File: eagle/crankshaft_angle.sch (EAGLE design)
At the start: 2 parts, among them U1 ATTINY25V-10PU

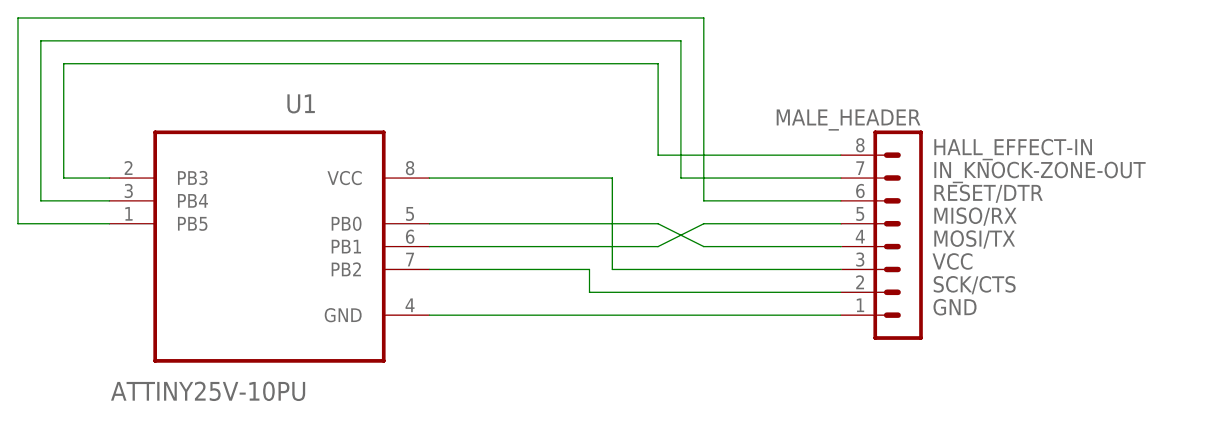
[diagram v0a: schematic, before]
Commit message: edit schematics
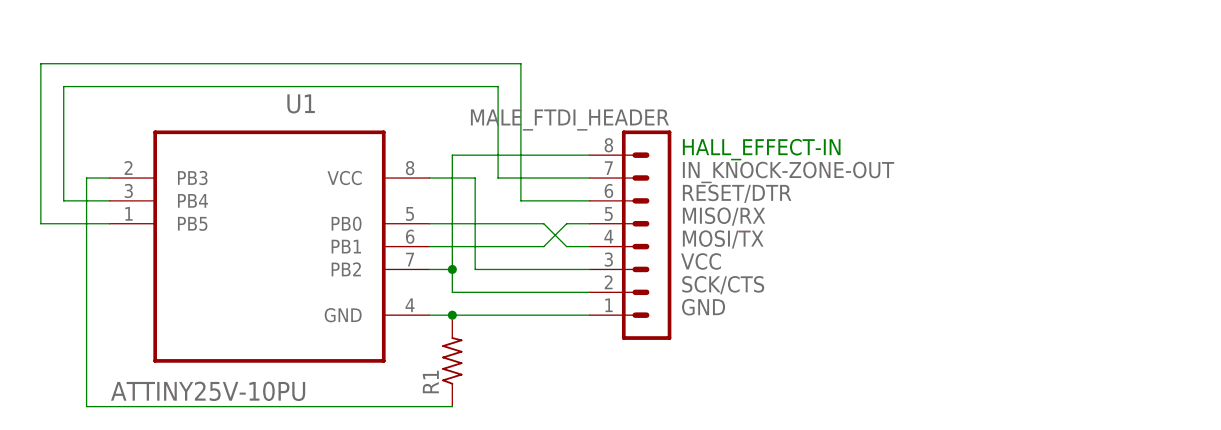
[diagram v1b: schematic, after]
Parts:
- removed MALE_HEADER: (no value), con-lstb:MA08-1
- added MALE_FTDI_HEADER: (no value), con-lstb:MA08-1
- added R1: (no value), rcl:R-US_0204/7
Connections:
- removed net HALL_EFFECT-IN: MALE_HEADER.8, U1.PB3
- new net N$1: R1.1, U1.PB3
- net GND: now also MALE_FTDI_HEADER.1, R1.2; no longer MALE_HEADER.1
- net IN_KNOCK-ZONE-OUT: now also MALE_FTDI_HEADER.7; no longer MALE_HEADER.7
- net MISO/RX: now also MALE_FTDI_HEADER.5; no longer MALE_HEADER.5
- net MOSI/TX: now also MALE_FTDI_HEADER.4; no longer MALE_HEADER.4
- net RESET/DTR: now also MALE_FTDI_HEADER.6; no longer MALE_HEADER.6
- net SCK/CTS: now also MALE_FTDI_HEADER.2, MALE_FTDI_HEADER.8; no longer MALE_HEADER.2
- net VCC: now also MALE_FTDI_HEADER.3; no longer MALE_HEADER.3
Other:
- note added: "HALL_EFFECT-IN"
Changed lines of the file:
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@@
 <part name="FRAME1" library="frames" deviceset="LETTER_L" device=""/>
 <part name="U1" library="Atmel_By_element14_Batch_1-00" deviceset="ATTINY25V-10PU" device=""/>
-<part name="MALE_HEADER" library="con-lstb" deviceset="MA08-1" device=""/>
+<part name="MALE_FTDI_HEADER" library="con-lstb" deviceset="MA08-1" device=""/>
+<part name="R1" library="rcl" deviceset="R-US_" device="0204/7"/>
 </parts>
 <sheets>
 <sheet>
 <plain>
+<text x="152.4" y="81.28" size="1.778" layer="91">HALL_EFFECT-IN</text>
 </plain>
 <instances>
@@
 <instance part="FRAME1" gate="G$2" x="139.7" y="-17.78"/>
 <instance part="U1" gate="A" x="106.68" y="73.66" rot="MR0"/>
-<instance part="MALE_HEADER" gate="1" x="177.8" y="71.12" rot="MR0"/>
+<instance part="MALE_FTDI_HEADER" gate="1" x="149.86" y="71.12" rot="MR0"/>
+<instance part="R1" gate="G$1" x="127" y="58.42" rot="R90"/>
 </instances>
 <busses>
@@
 <net name="SCK/CTS" class="0">
 <segment>
-<wire x1="170.18" y1="66.04" x2="142.24" y2="66.04" width="0.1524" layer="91"/>
-<wire x1="142.24" y1="66.04" x2="142.24" y2="68.58" width="0.1524" layer="91"/>
+<pinref part="MALE_FTDI_HEADER" gate="1" pin="8"/>
 <pinref part="U1" gate="A" pin="PB2"/>
-<wire x1="142.24" y1="68.58" x2="124.46" y2="68.58" width="0.1524" layer="91"/>
-<pinref part="MALE_HEADER" gate="1" pin="2"/>
-<label x="180.34" y="66.04" size="1.778" layer="95"/>
+<wire x1="127" y1="68.58" x2="124.46" y2="68.58" width="0.1524" layer="91"/>
+<wire x1="142.24" y1="81.28" x2="127" y2="81.28" width="0.1524" layer="91"/>
+<wire x1="127" y1="81.28" x2="127" y2="68.58" width="0.1524" layer="91"/>
+<wire x1="127" y1="68.58" x2="127" y2="66.04" width="0.1524" layer="91"/>
+<junction x="127" y="68.58"/>
+<pinref part="MALE_FTDI_HEADER" gate="1" pin="2"/>
+<wire x1="127" y1="66.04" x2="142.24" y2="66.04" width="0.1524" layer="91"/>
+<label x="152.4" y="66.04" size="1.778" layer="95"/>
 </segment>
 </net>
 <net name="RESET/DTR" class="0">
 <segment>
-<wire x1="154.94" y1="76.2" x2="154.94" y2="96.52" width="0.1524" layer="91"/>
-<wire x1="154.94" y1="96.52" x2="78.74" y2="96.52" width="0.1524" layer="91"/>
-<wire x1="78.74" y1="96.52" x2="78.74" y2="73.66" width="0.1524" layer="91"/>
+<wire x1="134.62" y1="76.2" x2="134.62" y2="91.44" width="0.1524" layer="91"/>
+<wire x1="134.62" y1="91.44" x2="81.28" y2="91.44" width="0.1524" layer="91"/>
+<wire x1="81.28" y1="91.44" x2="81.28" y2="73.66" width="0.1524" layer="91"/>
 <pinref part="U1" gate="A" pin="PB5"/>
-<wire x1="78.74" y1="73.66" x2="88.9" y2="73.66" width="0.1524" layer="91"/>
-<pinref part="MALE_HEADER" gate="1" pin="6"/>
-<wire x1="170.18" y1="76.2" x2="154.94" y2="76.2" width="0.1524" layer="91"/>
-<label x="180.34" y="76.2" size="1.778" layer="95"/>
+<wire x1="81.28" y1="73.66" x2="88.9" y2="73.66" width="0.1524" layer="91"/>
+<pinref part="MALE_FTDI_HEADER" gate="1" pin="6"/>
+<wire x1="142.24" y1="76.2" x2="134.62" y2="76.2" width="0.1524" layer="91"/>
+<label x="152.4" y="76.2" size="1.778" layer="95"/>
 </segment>
 </net>
@@
 <segment>
 <pinref part="U1" gate="A" pin="PB4"/>
-<wire x1="88.9" y1="76.2" x2="81.28" y2="76.2" width="0.1524" layer="91"/>
-<wire x1="81.28" y1="76.2" x2="81.28" y2="93.98" width="0.1524" layer="91"/>
-<wire x1="81.28" y1="93.98" x2="152.4" y2="93.98" width="0.1524" layer="91"/>
-<wire x1="152.4" y1="93.98" x2="152.4" y2="78.74" width="0.1524" layer="91"/>
-<pinref part="MALE_HEADER" gate="1" pin="7"/>
-<wire x1="152.4" y1="78.74" x2="170.18" y2="78.74" width="0.1524" layer="91"/>
-<label x="180.34" y="78.74" size="1.778" layer="95"/>
-</segment>
-</net>
-<net name="HALL_EFFECT-IN" class="0">
-<segment>
-<pinref part="MALE_HEADER" gate="1" pin="8"/>
-<wire x1="170.18" y1="81.28" x2="149.86" y2="81.28" width="0.1524" layer="91"/>
-<wire x1="149.86" y1="81.28" x2="149.86" y2="91.44" width="0.1524" layer="91"/>
-<wire x1="149.86" y1="91.44" x2="83.82" y2="91.44" width="0.1524" layer="91"/>
-<wire x1="83.82" y1="91.44" x2="83.82" y2="78.74" width="0.1524" layer="91"/>
-<pinref part="U1" gate="A" pin="PB3"/>
-<wire x1="83.82" y1="78.74" x2="88.9" y2="78.74" width="0.1524" layer="91"/>
-<label x="180.34" y="81.28" size="1.778" layer="95"/>
+<wire x1="88.9" y1="76.2" x2="83.82" y2="76.2" width="0.1524" layer="91"/>
+<wire x1="83.82" y1="76.2" x2="83.82" y2="88.9" width="0.1524" layer="91"/>
+<wire x1="83.82" y1="88.9" x2="132.08" y2="88.9" width="0.1524" layer="91"/>
+<wire x1="132.08" y1="88.9" x2="132.08" y2="78.74" width="0.1524" layer="91"/>
+<pinref part="MALE_FTDI_HEADER" gate="1" pin="7"/>
+<wire x1="132.08" y1="78.74" x2="142.24" y2="78.74" width="0.1524" layer="91"/>
+<label x="152.4" y="78.74" size="1.778" layer="95"/>
 </segment>
 </net>
@@
 <segment>
 <pinref part="U1" gate="A" pin="GND"/>
-<pinref part="MALE_HEADER" gate="1" pin="1"/>
-<wire x1="124.46" y1="63.5" x2="170.18" y2="63.5" width="0.1524" layer="91"/>
-<label x="180.34" y="63.5" size="1.778" layer="95"/>
+<pinref part="MALE_FTDI_HEADER" gate="1" pin="1"/>
+<wire x1="124.46" y1="63.5" x2="127" y2="63.5" width="0.1524" layer="91"/>
+<label x="152.4" y="63.5" size="1.778" layer="95"/>
+<pinref part="R1" gate="G$1" pin="2"/>
+<wire x1="127" y1="63.5" x2="142.24" y2="63.5" width="0.1524" layer="91"/>
+<junction x="127" y="63.5"/>
 </segment>
 </net>
@@
 <segment>
 <pinref part="U1" gate="A" pin="VCC"/>
-<wire x1="124.46" y1="78.74" x2="144.78" y2="78.74" width="0.1524" layer="91"/>
-<wire x1="144.78" y1="78.74" x2="144.78" y2="68.58" width="0.1524" layer="91"/>
-<pinref part="MALE_HEADER" gate="1" pin="3"/>
-<wire x1="144.78" y1="68.58" x2="170.18" y2="68.58" width="0.1524" layer="91"/>
-<label x="180.34" y="68.58" size="1.778" layer="95"/>
+<wire x1="124.46" y1="78.74" x2="129.54" y2="78.74" width="0.1524" layer="91"/>
+<wire x1="129.54" y1="78.74" x2="129.54" y2="68.58" width="0.1524" layer="91"/>
+<pinref part="MALE_FTDI_HEADER" gate="1" pin="3"/>
+<wire x1="129.54" y1="68.58" x2="142.24" y2="68.58" width="0.1524" layer="91"/>
+<label x="152.4" y="68.58" size="1.778" layer="95"/>
 </segment>
 </net>
@@
 <segment>
 <pinref part="U1" gate="A" pin="PB0"/>
-<wire x1="124.46" y1="73.66" x2="149.86" y2="73.66" width="0.1524" layer="91"/>
-<wire x1="149.86" y1="73.66" x2="154.94" y2="71.12" width="0.1524" layer="91"/>
-<pinref part="MALE_HEADER" gate="1" pin="4"/>
-<wire x1="154.94" y1="71.12" x2="170.18" y2="71.12" width="0.1524" layer="91"/>
-<label x="180.34" y="71.12" size="1.778" layer="95"/>
+<wire x1="124.46" y1="73.66" x2="137.16" y2="73.66" width="0.1524" layer="91"/>
+<wire x1="137.16" y1="73.66" x2="139.7" y2="71.12" width="0.1524" layer="91"/>
+<pinref part="MALE_FTDI_HEADER" gate="1" pin="4"/>
+<wire x1="139.7" y1="71.12" x2="142.24" y2="71.12" width="0.1524" layer="91"/>
+<label x="152.4" y="71.12" size="1.778" layer="95"/>
 </segment>
 </net>
 <net name="MISO/RX" class="0">
 <segment>
-<pinref part="MALE_HEADER" gate="1" pin="5"/>
-<wire x1="170.18" y1="73.66" x2="154.94" y2="73.66" width="0.1524" layer="91"/>
-<wire x1="154.94" y1="73.66" x2="149.86" y2="71.12" width="0.1524" layer="91"/>
+<pinref part="MALE_FTDI_HEADER" gate="1" pin="5"/>
+<wire x1="142.24" y1="73.66" x2="139.7" y2="73.66" width="0.1524" layer="91"/>
+<wire x1="139.7" y1="73.66" x2="137.16" y2="71.12" width="0.1524" layer="91"/>
 <pinref part="U1" gate="A" pin="PB1"/>
-<wire x1="149.86" y1="71.12" x2="124.46" y2="71.12" width="0.1524" layer="91"/>
-<label x="180.34" y="73.66" size="1.778" layer="95"/>
+<wire x1="137.16" y1="71.12" x2="124.46" y2="71.12" width="0.1524" layer="91"/>
+<label x="152.4" y="73.66" size="1.778" layer="95"/>
 </segment>
 </net>
+<net name="N$1" class="0">
+<segment>
+<pinref part="U1" gate="A" pin="PB3"/>
+<wire x1="88.9" y1="78.74" x2="86.36" y2="78.74" width="0.1524" layer="91"/>
+<wire x1="86.36" y1="78.74" x2="86.36" y2="53.34" width="0.1524" layer="91"/>
+<pinref part="R1" gate="G$1" pin="1"/>
+<wire x1="86.36" y1="53.34" x2="127" y2="53.34" width="0.1524" layer="91"/>
+</segment>
+</net>
